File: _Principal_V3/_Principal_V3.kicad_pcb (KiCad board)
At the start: 2 copper layers, 73 parts, among them J1 CAN, J10 UART, J11 I2C, J12 NEXTION, J2 ENCODEUR_G, J3 ENCODEUR_D, J4 CAN, J5 MOTOR_D, J6 BATT, J7 MOTOR_G, J8 FAN, J9 FAN, Q1 SI2302S, Q2 SI2302S, Q3 SI2302S, Q4 SI2302S, Q5 SI2302S, Q6 SI2302S, U1 4504, U2 SN65HVD232, U3 Teensy3.6

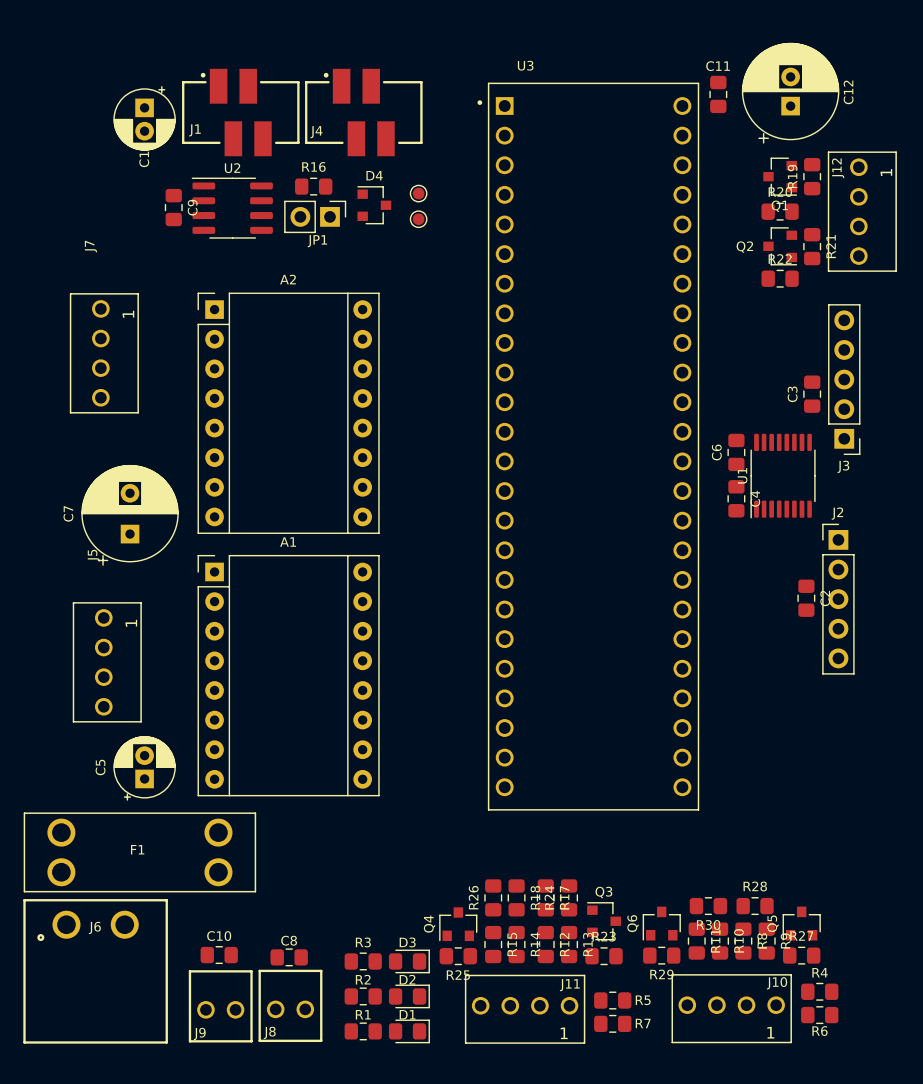
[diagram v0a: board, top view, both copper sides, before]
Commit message: lots of stuf
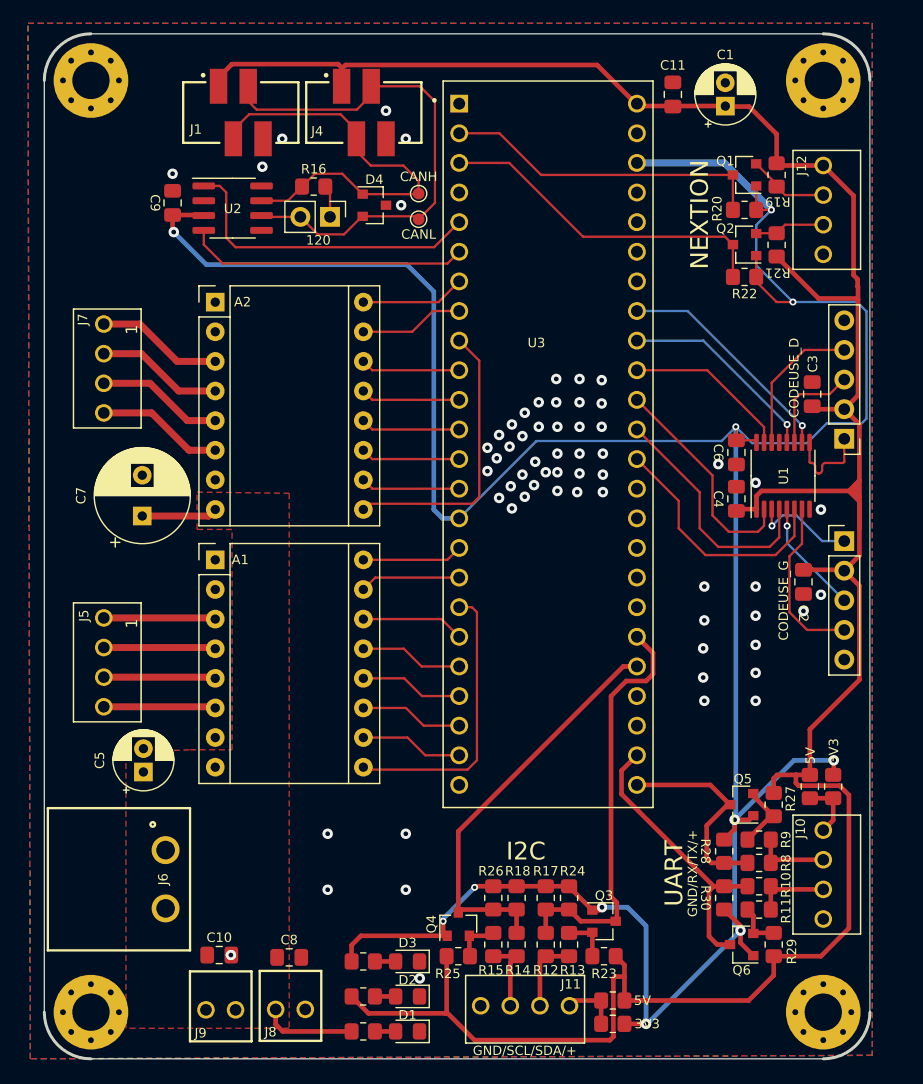
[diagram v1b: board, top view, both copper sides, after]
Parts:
- removed C12: 10u, Capacitor_THT:CP_Radial_D8.0mm_P2.50mm
- removed F1: 10A, AREA_lib_composant:FUSE_3557-2
- added H1: MountingHole_Pad, MountingHole:MountingHole_3.2mm_M3_Pad_Via, F.Cu at (67.4, 134.5)
- added H2: MountingHole_Pad, MountingHole:MountingHole_3.2mm_M3_Pad_Via, F.Cu at (67.4, 54.6)
- added H3: MountingHole_Pad, MountingHole:MountingHole_3.2mm_M3_Pad_Via, F.Cu at (130.2, 54.6)
- added H4: MountingHole_Pad, MountingHole:MountingHole_3.2mm_M3_Pad_Via, F.Cu at (130.2, 134.5)
- 3V3: renamed from R6; footprint Resistor_SMD:R_0805_2012Metric_Pad1.15x1.40mm_HandSolder -> Resistor_SMD:R_0805_2012Metric_Pad1.20x1.40mm_HandSolder
- 3V3: renamed from R7; footprint Resistor_SMD:R_0805_2012Metric_Pad1.15x1.40mm_HandSolder -> Resistor_SMD:R_0805_2012Metric_Pad1.20x1.40mm_HandSolder
- 5V: renamed from R4; footprint Resistor_SMD:R_0805_2012Metric_Pad1.15x1.40mm_HandSolder -> Resistor_SMD:R_0805_2012Metric_Pad1.20x1.40mm_HandSolder
- 5V: renamed from R5; footprint Resistor_SMD:R_0805_2012Metric_Pad1.15x1.40mm_HandSolder -> Resistor_SMD:R_0805_2012Metric_Pad1.20x1.40mm_HandSolder
- C10, C11, C2, C3, C4, C6, C8, C9: footprint Capacitor_SMD:C_0805_2012Metric_Pad1.15x1.40mm_HandSolder -> Capacitor_SMD:C_0805_2012Metric_Pad1.18x1.45mm_HandSolder
- R1, R10, R11, R12, R13, R14, R15, R16, R17, R18, R19, R2, R20, R21, R22, R23, R24, R25, R26, R27, R28, R29, R3, R30, R8, R9: footprint Resistor_SMD:R_0805_2012Metric_Pad1.15x1.40mm_HandSolder -> Resistor_SMD:R_0805_2012Metric_Pad1.20x1.40mm_HandSolder
- U3: value Teensy3.6 -> DEV-14058; footprint AREA_lib_composant:TEENSY_3.6 -> AREA_lib_composant:MODULE_DEV-14058
- moved C1 49.8 mm to (121.8, 56.8), turned to 90 degrees
- moved 3V3 19.6 mm to (131.1, 115.2), turned to -90 degrees
- moved 5V 17.6 mm to (129.1, 115.2), turned to -90 degrees
- moved J10 13.7 mm to (130.2, 122.7), turned to 90 degrees
- moved R27 13.2 mm to (126.0, 116.7), turned to 90 degrees
- moved Q5 11.4 mm to (123.2, 116.7), turned to 180 degrees
- moved R29 9.65 mm to (126.0, 128.7), turned to -90 degrees
- moved R9 8.72 mm to (124.7, 119.7), turned to 0 degrees
- moved J6 7.16 mm to (73.8, 123.1), turned to -90 degrees
- moved Q6 7.08 mm to (123.2, 128.7), turned to 180 degrees
- moved R8 6.83 mm to (124.7, 121.7), turned to 0 degrees
- moved R11 5.99 mm to (124.7, 125.7), turned to 0 degrees
- moved R10 5.77 mm to (124.7, 123.7), turned to 0 degrees
- moved R28 5.40 mm to (121.7, 120.7), turned to 90 degrees
- moved U3 3.91 mm to (106.6, 85.8)
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- renumbered JP1 to 120, TP1 to CANH, TP2 to CANL, J3 to CODEUSE_D, J2 to CODEUSE_G
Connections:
- A1 pad 2: Net-(A1-Pad2) -> unconnected-(A1-Pad2)
- A2 pad 2: Net-(A2-Pad2) -> unconnected-(A2-Pad2)
- J6 pad 1: Net-(F1-Pad2) -> +24V
- U2 pad 5: Net-(U2-Pad5) -> unconnected-(U2-Pad5)
- U2 pad 8: Net-(U2-Pad8) -> unconnected-(U2-Pad8)
- U3 pad 15: Net-(U3-Pad15) -> +3V3
- U3 pad 24: Net-(U3-Pad24) -> unconnected-(U3-Pad24)
- U3 pad 25: Net-(U3-Pad25) -> /TX
- U3 pad 26: Net-(U3-Pad26) -> /RX
- U3 pad 27: GND -> unconnected-(U3-Pad27)
- U3 pad 28: Net-(U3-Pad28) -> unconnected-(U3-Pad28)
- U3 pad 29: Net-(U3-Pad29) -> /SCL
- U3 pad 30: /TX -> /SDA
- U3 pad 31: /RX -> unconnected-(U3-Pad31)
- U3 pad 32: /CHANNEL_B_G -> unconnected-(U3-Pad32)
- U3 pad 33: /CHANNEL_A_G -> unconnected-(U3-Pad33)
- U3 pad 34: /CHANNEL_IDX_G -> GND
- U3 pad 35: /CHANNEL_B_D -> unconnected-(U3-Pad35)
- U3 pad 36: /CHANNEL_A_D -> /CHANNEL_IDX_G
- U3 pad 37: /CHANNEL_IDX_D -> /CHANNEL_A_G
- U3 pad 38: Net-(U3-Pad38) -> /CHANNEL_B_G
- U3 pad 39: GND -> /CHANNEL_IDX_D
- U3 pad 4: Net-(U3-Pad4) -> unconnected-(U3-Pad4)
- U3 pad 40: Net-(U3-Pad40) -> /CHANNEL_A_D
- U3 pad 41: Net-(U3-Pad41) -> /CHANNEL_B_D
- U3 pad 42: Net-(U3-Pad42) -> unconnected-(U3-Pad42)
- U3 pad 43: Net-(U3-Pad43) -> unconnected-(U3-Pad43)
- U3 pad 44: Net-(U3-Pad44) -> unconnected-(U3-Pad44)
- U3 pad 45: /SDA -> unconnected-(U3-Pad45)
- U3 pad 46: /SCL -> +3V3
- U3 pad 47: Net-(U3-Pad47) -> GND
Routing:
- net +3V3: track 0.00 -> 258.4 mm, vias 0 -> 11
- net +5V: track 0.00 -> 236.5 mm
- net /CANL: track 0.00 -> 45.0 mm
- net /CANH: track 0.00 -> 36.9 mm
- net /SDA: track 0.00 -> 36.1 mm
- net /SCL: track 0.00 -> 35.2 mm
- net /NEXTION_TX: track 0.00 -> 29.1 mm
- net /NEXTION_RX: track 0.00 -> 27.9 mm
- net /TX_CAN: track 0.00 -> 27.3 mm
- net /EN_D: track 0.00 -> 24.6 mm
- net /RX: track 0.00 -> 24.5 mm
- net /EN_G: track 0.00 -> 24.5 mm
- net /RX_CAN: track 0.00 -> 24.2 mm
- net /CHANNEL_IDX_G: track 0.00 -> 21.3 mm
- net /CHANNEL_A_G: track 0.00 -> 20.9 mm
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- added copper zone on F.Cu, net +24V
- added copper zone on B.Cu, net GND
- added copper zone on F.Cu, net GND
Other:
- board outline added: 70.8 x 87.9 mm
- net class Default removed
- board text added: "GND/RX/TX/+"
- board text added: "GND/SCL/SDA/+"
- board text added: "I2C"
- board text added: "NEXTION"
- board text added: "UART"
